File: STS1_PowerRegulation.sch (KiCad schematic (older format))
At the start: 16 parts, among them U2 TPS61288

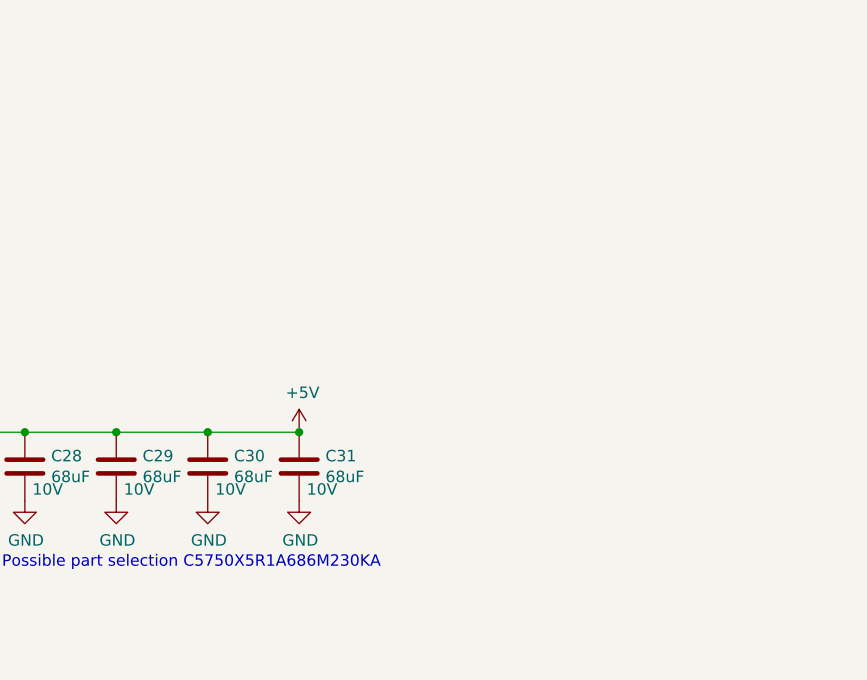
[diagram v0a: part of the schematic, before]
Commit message: final version1
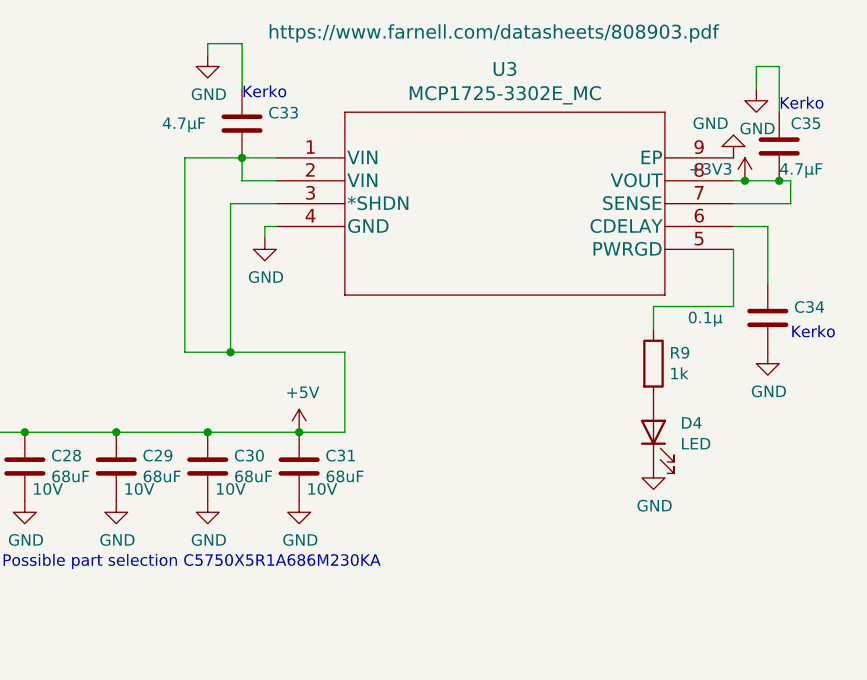
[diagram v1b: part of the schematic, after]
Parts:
- added C33, C35: 4.7µF, Capacitor_SMD:C_0805_2012Metric, symbol Device:C
- added C34: 0.1µ, Capacitor_SMD:C_0805_2012Metric, symbol Device:C
- added D4: LED, LED_SMD:LED_0805_2012Metric, symbol Device:LED
- added R9: 1k, Resistor_SMD:R_0805_2012Metric, symbol Device:R
- added U3: MCP1725-3302E_MC, STS1_3V3:MCP1725-3302E&slash_MC, symbol STS1_3V3:MCP1725-3302E_MC
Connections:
- net +5V: now also C33.2, U3.1 (VIN), U3.2 (VIN), U3.3 (*SHDN)
- net GND: now also C33.1, C34.2, C35.1, D4.1 (K), U3.4 (GND), U3.9 (EP)
- new net: C34.1, U3.6 (CDELAY)
- new net: R9.1, U3.5 (PWRGD)
- new net: D4.2 (A), R9.2
- new net +3V3: C35.2, U3.7 (SENSE), U3.8 (VOUT)
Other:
- note added: "Kerko\n"
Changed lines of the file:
@@
 $Descr A4 11693 8268
 encoding utf-8
-Sheet 5 5
+Sheet 4 6
 Title ""
 Date ""
@@
 Text Notes 7700 3200 0    50   ~ 0
 Possible part selection C5750X5R1A686M230KA
+$Comp
+L STS1_3V3:MCP1725-3302E_MC U3
+U 1 1 6199338A
+P 8900 1400
+F 0 "U3" H 9900 1787 60  0000 C CNN
+F 1 "MCP1725-3302E_MC" H 9900 1681 60  0000 C CNN
+F 2 "STS1_3V3:MCP1725-3302E&slash_MC" H 9900 1640 60  0001 C CNN
+F 3 "https://www.farnell.com/datasheets/808903.pdf" H 9850 1950 60  0000 C CNN
+	1    8900 1400
+	1    0    0    -1
+$EndComp
+Wire Wire Line
+	9000 2600 9200 2600
+Wire Wire Line
+	9200 2600 9200 2250
+Wire Wire Line
+	9200 2250 8700 2250
+Wire Wire Line
+	8500 2250 8500 1400
+Wire Wire Line
+	8500 1400 8750 1400
+$Comp
+L Device:C C33
+U 1 1 61995988
+P 8750 1250
+F 0 "C33" H 8865 1296 50  0000 L CNN
+F 1 "4.7µF" H 8400 1250 50  0000 L CNN
+F 2 "Capacitor_SMD:C_0805_2012Metric" H 8788 1100 50  0001 C CNN
+F 3 "~" H 8750 1250 50  0001 C CNN
+	1    8750 1250
+	1    0    0    -1
+$EndComp
+Connection ~ 8750 1400
+Wire Wire Line
+	8750 1400 8900 1400
+$Comp
+L power:GND #PWR023
+U 1 1 619967E2
+P 8600 950
+F 0 "#PWR023" H 8600 700 50  0001 C CNN
+F 1 "GND" H 8605 777 50  0000 C CNN
+F 2 "" H 8600 950 50  0001 C CNN
+F 3 "" H 8600 950 50  0001 C CNN
+	1    8600 950
+	1    0    0    -1
+$EndComp
+Wire Wire Line
+	8750 1100 8750 900
+Wire Wire Line
+	8750 900  8600 900
+Wire Wire Line
+	8600 900  8600 950
+Wire Wire Line
+	8750 1400 8750 1500
+Wire Wire Line
+	8750 1500 8900 1500
+Wire Wire Line
+	8700 2250 8700 1600
+Wire Wire Line
+	8700 1600 8900 1600
+Connection ~ 8700 2250
+Wire Wire Line
+	8700 2250 8500 2250
+$Comp
+L power:GND #PWR024
+U 1 1 61999442
+P 8850 1750
+F 0 "#PWR024" H 8850 1500 50  0001 C CNN
+F 1 "GND" H 8855 1577 50  0000 C CNN
+F 2 "" H 8850 1750 50  0001 C CNN
+F 3 "" H 8850 1750 50  0001 C CNN
+	1    8850 1750
+	1    0    0    -1
+$EndComp
+Wire Wire Line
+	8900 1700 8850 1700
+Wire Wire Line
+	8850 1700 8850 1750
+Wire Wire Line
+	10900 1600 11150 1600
+Wire Wire Line
+	11150 1600 11150 1500
+Wire Wire Line
+	11150 1500 11100 1500
+$Comp
+L Device:C C35
+U 1 1 619A5F9B
+P 11100 1350
+F 0 "C35" H 11150 1450 50  0000 L CNN
+F 1 "4.7µF" H 11100 1250 50  0000 L CNN
+F 2 "Capacitor_SMD:C_0805_2012Metric" H 11138 1200 50  0001 C CNN
+F 3 "~" H 11100 1350 50  0001 C CNN
+	1    11100 1350
+	1    0    0    -1
+$EndComp
+Connection ~ 11100 1500
+Wire Wire Line
+	11100 1500 10950 1500
+$Comp
+L power:GND #PWR027
+U 1 1 619A6A54
+P 11000 1100
+F 0 "#PWR027" H 11000 850 50  0001 C CNN
+F 1 "GND" H 11005 927 50  0000 C CNN
+F 2 "" H 11000 1100 50  0001 C CNN
+F 3 "" H 11000 1100 50  0001 C CNN
+	1    11000 1100
+	1    0    0    -1
+$EndComp
+Wire Wire Line
+	11100 1200 11100 1000
+Wire Wire Line
+	11100 1000 11000 1000
+Wire Wire Line
+	11000 1000 11000 1100
+Text Notes 11100 1200 0    50   ~ 0
+Kerko\n
+$Comp
+L Device:C C34
+U 1 1 6197D6D8
+P 11050 2100
+F 0 "C34" H 11165 2146 50  0000 L CNN
+F 1 "0.1µ" H 10700 2100 50  0000 L CNN
+F 2 "Capacitor_SMD:C_0805_2012Metric" H 11088 1950 50  0001 C CNN
+F 3 "~" H 11050 2100 50  0001 C CNN
+	1    11050 2100
+	1    0    0    -1
+$EndComp
+$Comp
+L power:GND #PWR028
+U 1 1 6197E02C
+P 11050 2250
+F 0 "#PWR028" H 11050 2000 50  0001 C CNN
+F 1 "GND" H 11055 2077 50  0000 C CNN
+F 2 "" H 11050 2250 50  0001 C CNN
+F 3 "" H 11050 2250 50  0001 C CNN
+	1    11050 2250
+	1    0    0    -1
+$EndComp
+Wire Wire Line
+	10900 1700 11050 1700
+Wire Wire Line
+	11050 1700 11050 1950
+$Comp
+L Device:R R9
+U 1 1 6197F7C2
+P 10550 2300
+F 0 "R9" H 10620 2346 50  0000 L CNN
+F 1 "1k" H 10620 2255 50  0000 L CNN
+F 2 "Resistor_SMD:R_0805_2012Metric" V 10480 2300 50  0001 C CNN
+F 3 "~" H 10550 2300 50  0001 C CNN
+	1    10550 2300
+	1    0    0    -1
+$EndComp
+Wire Wire Line
+	10550 2150 10550 2050
+Wire Wire Line
+	10550 2050 10900 2050
+Wire Wire Line
+	10900 2050 10900 1800
+$Comp
+L power:GND #PWR025
+U 1 1 6198107B
+P 10550 2750
+F 0 "#PWR025" H 10550 2500 50  0001 C CNN
+F 1 "GND" H 10555 2577 50  0000 C CNN
+F 2 "" H 10550 2750 50  0001 C CNN
+F 3 "" H 10550 2750 50  0001 C CNN
+	1    10550 2750
+	1    0    0    -1
+$EndComp
+$Comp
+L Device:LED D4
+U 1 1 61981BA6
+P 10550 2600
+F 0 "D4" V 10589 2482 50  0000 R CNN
+F 1 "LED" V 10498 2482 50  0000 R CNN
+F 2 "LED_SMD:LED_0805_2012Metric" H 10550 2600 50  0001 C CNN
+F 3 "~" H 10550 2600 50  0001 C CNN
+	1    10550 2600
+	0    -1   -1   0
+$EndComp
+Text Notes 8750 1150 0    50   ~ 0
+Kerko\n
+Text Notes 11150 2200 0    50   ~ 0
+Kerko\n
+$Comp
+L power:+3V3 #PWR026
+U 1 1 619903E6
+P 10950 1500
+F 0 "#PWR026" H 10950 1350 50  0001 C CNN
+F 1 "+3V3" H 10800 1550 50  0000 C CNN
+F 2 "" H 10950 1500 50  0001 C CNN
+F 3 "" H 10950 1500 50  0001 C CNN
+	1    10950 1500
+	1    0    0    -1
+$EndComp
+Connection ~ 10950 1500
+Wire Wire Line
+	10950 1500 10900 1500
+$Comp
+L power:GND #PWR0138
+U 1 1 61993623
+P 10900 1400
+F 0 "#PWR0138" H 10900 1150 50  0001 C CNN
+F 1 "GND" H 11000 1250 50  0000 C CNN
+F 2 "" H 10900 1400 50  0001 C CNN
+F 3 "" H 10900 1400 50  0001 C CNN
+	1    10900 1400
+	-1   0    0    1
+$EndComp
 $EndSCHEMATC
